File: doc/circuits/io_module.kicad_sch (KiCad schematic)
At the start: 11 parts, among them SW1 SW_MEC_5G, SW2 SW_DPDT_x2, SW3 SW_MEC_5G, U1 RC1602A-GHW-ESX, U2 74LS04, U3 74HC595

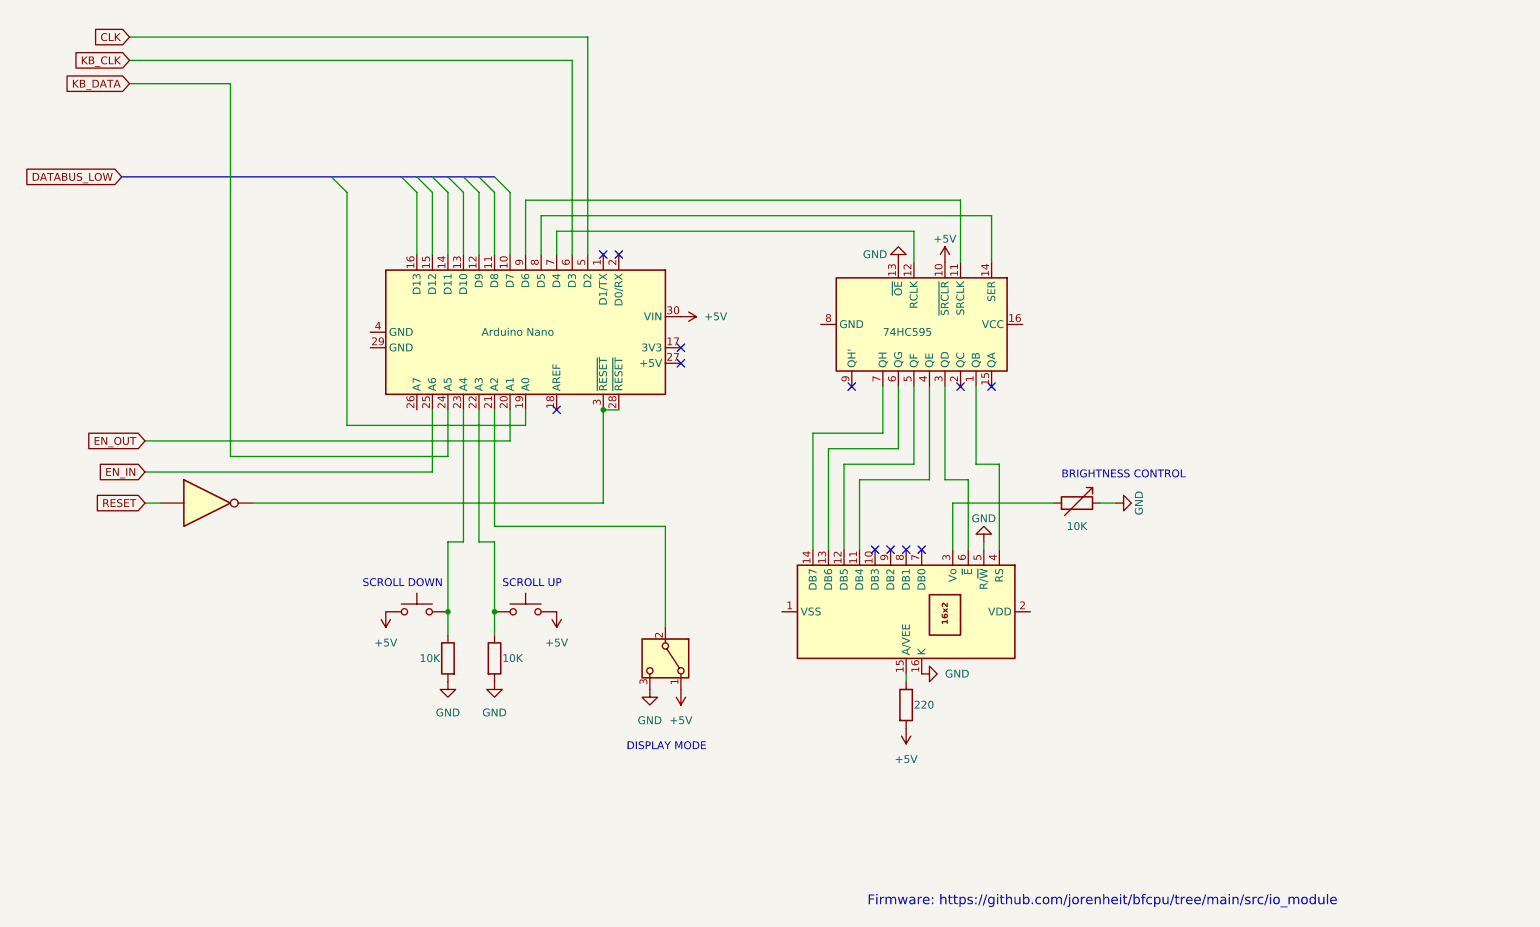
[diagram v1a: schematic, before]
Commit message: documentation
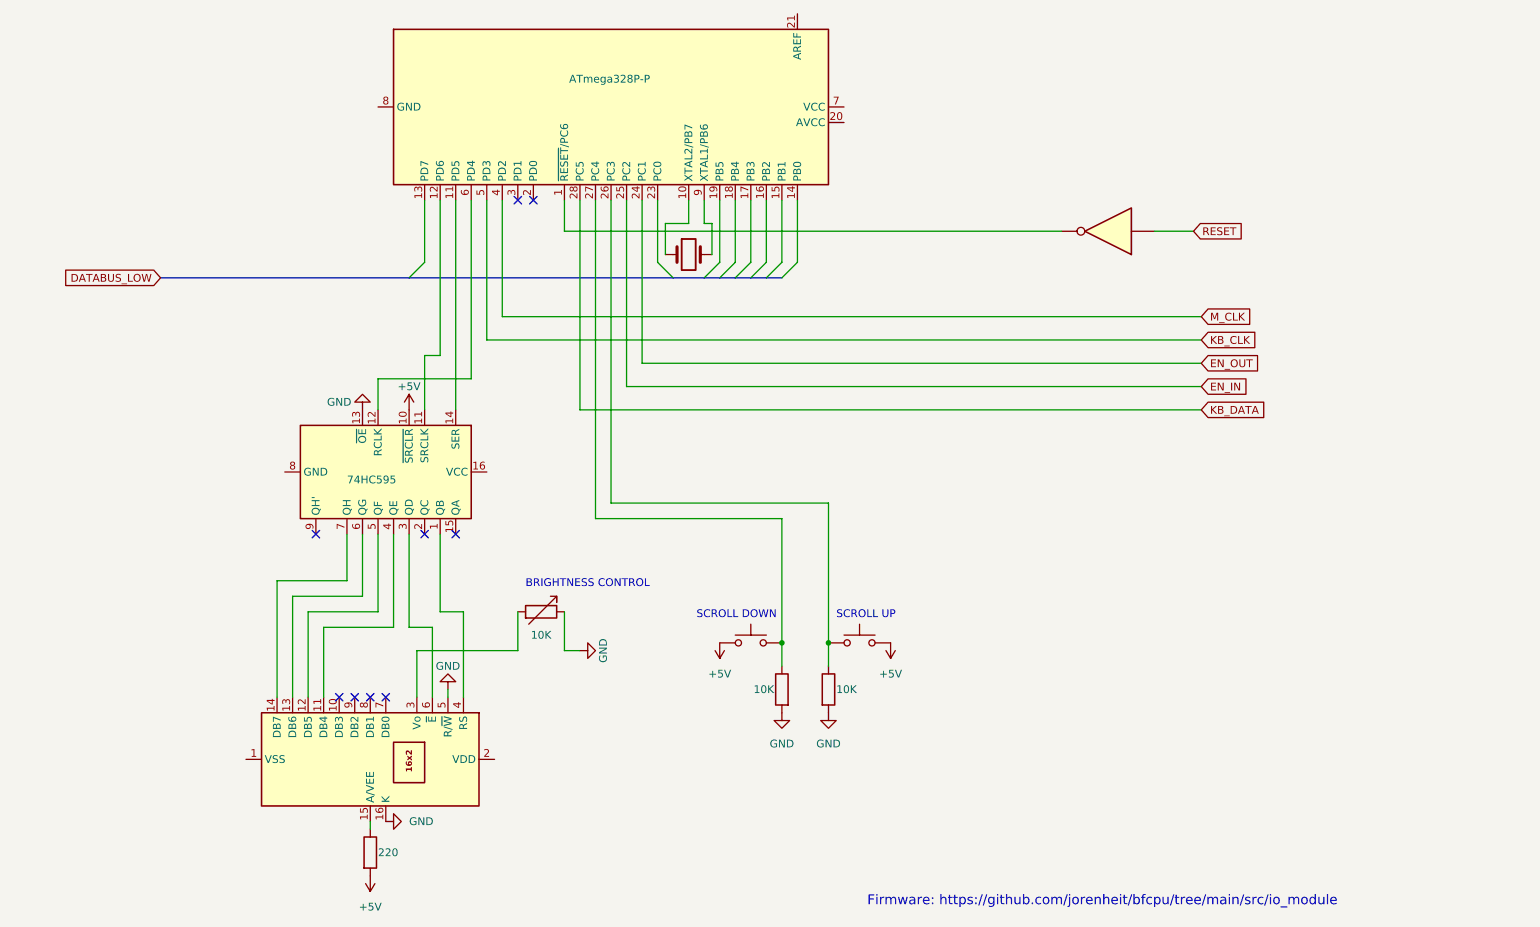
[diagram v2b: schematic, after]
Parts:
- removed A2: Arduino Nano, Module:Arduino_Nano, symbol MCU_Module:Arduino_Nano_v3.x
- removed SW2: SW_DPDT_x2, symbol Switch:SW_DPDT_x2
- added U4: ATmega328P-P, Package_DIP:DIP-28_W7.62mm, symbol MCU_Microchip_ATmega:ATmega328P-P
- added Y1: Crystal, symbol Device:Crystal
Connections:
- net EN_IN: now also U4.25 (PC2)
- net EN_OUT: now also U4.24 (PC1)
- net KB_CLK: now also U4.5 (PD3)
- net KB_DATA: now also U4.28 (PC5)
- net at U3.11 (SRCLK): now also U4.12 (PD6)
- net at U3.12 (RCLK): now also U4.6 (PD4)
- net at U3.14 (SER): now also U4.11 (PD5)
- net at R1.1, SW1.1 (A), SW1.2 (A): now also U4.27 (PC4)
- net at U2.2: now also U4.1 (~{RESET}/PC6)
- net at R2.1, SW3.1 (A), SW3.2 (A): now also U4.26 (PC3)
- new net: U4.10 (XTAL2/PB7), Y1.1
- new net: U4.22 (GND), U4.8 (GND)
- new net: U4.9 (XTAL1/PB6), Y1.2
- new net M_CLK: U4.4 (PD2)
- no-connect marks 12 -> 9
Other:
- note removed: "DISPLAY MODE"
